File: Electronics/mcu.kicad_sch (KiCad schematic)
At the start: 32 parts, among them J2 OLED_CONN, J3 UART_CONN, SW2 PEC12, SW4 MCU_EN, U1 ESP32-C4FH4, Y1 40MHz

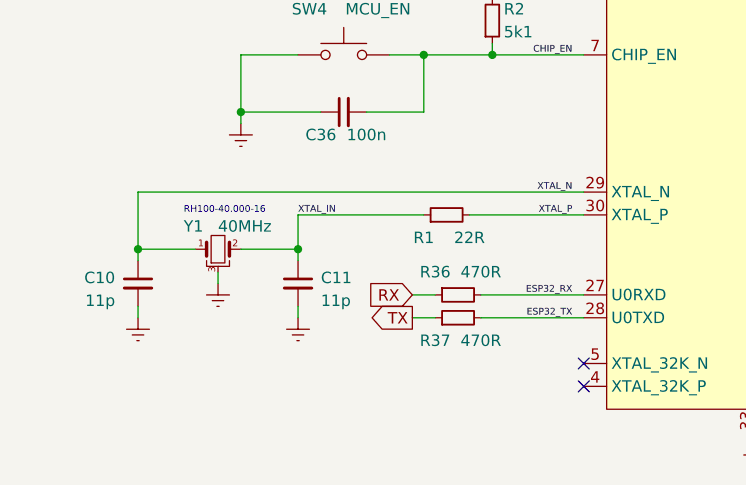
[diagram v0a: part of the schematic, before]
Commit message: Fixed crystal
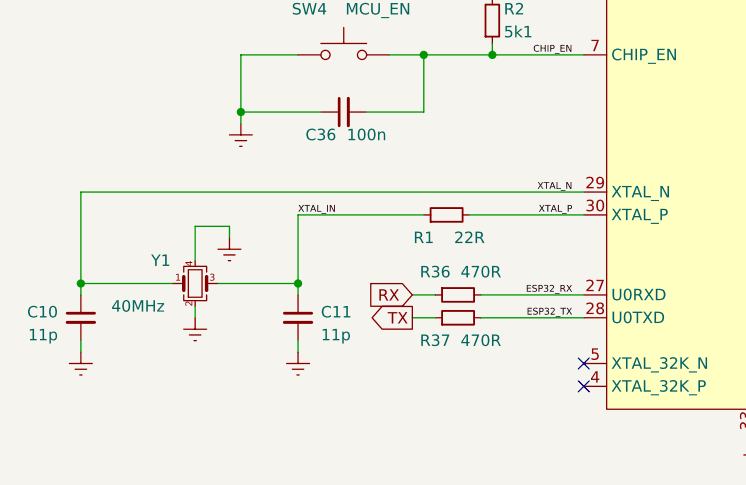
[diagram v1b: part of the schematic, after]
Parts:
- removed Y1: 40MHz, Crystal:Crystal_SMD_2520-4Pin_2.5x2.0mm, symbol Device:Crystal_GND3_Small
- added Y1: 40MHz, Crystal:Crystal_SMD_3225-4Pin_3.2x2.5mm, symbol Device:Crystal_GND24_Small
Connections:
- net Earth: now also Y1.2, Y1.4
- net XTAL_IN: now also Y1.3
- net XTAL_N: now also Y1.1
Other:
- note removed: "RH100-40.000-16"
- moved on the sheet: C10, C11
